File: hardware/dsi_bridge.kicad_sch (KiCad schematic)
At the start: 2 parts, among them J11 Conn_01x20_MountingPin, J12 Conn_01x20_MountingPin

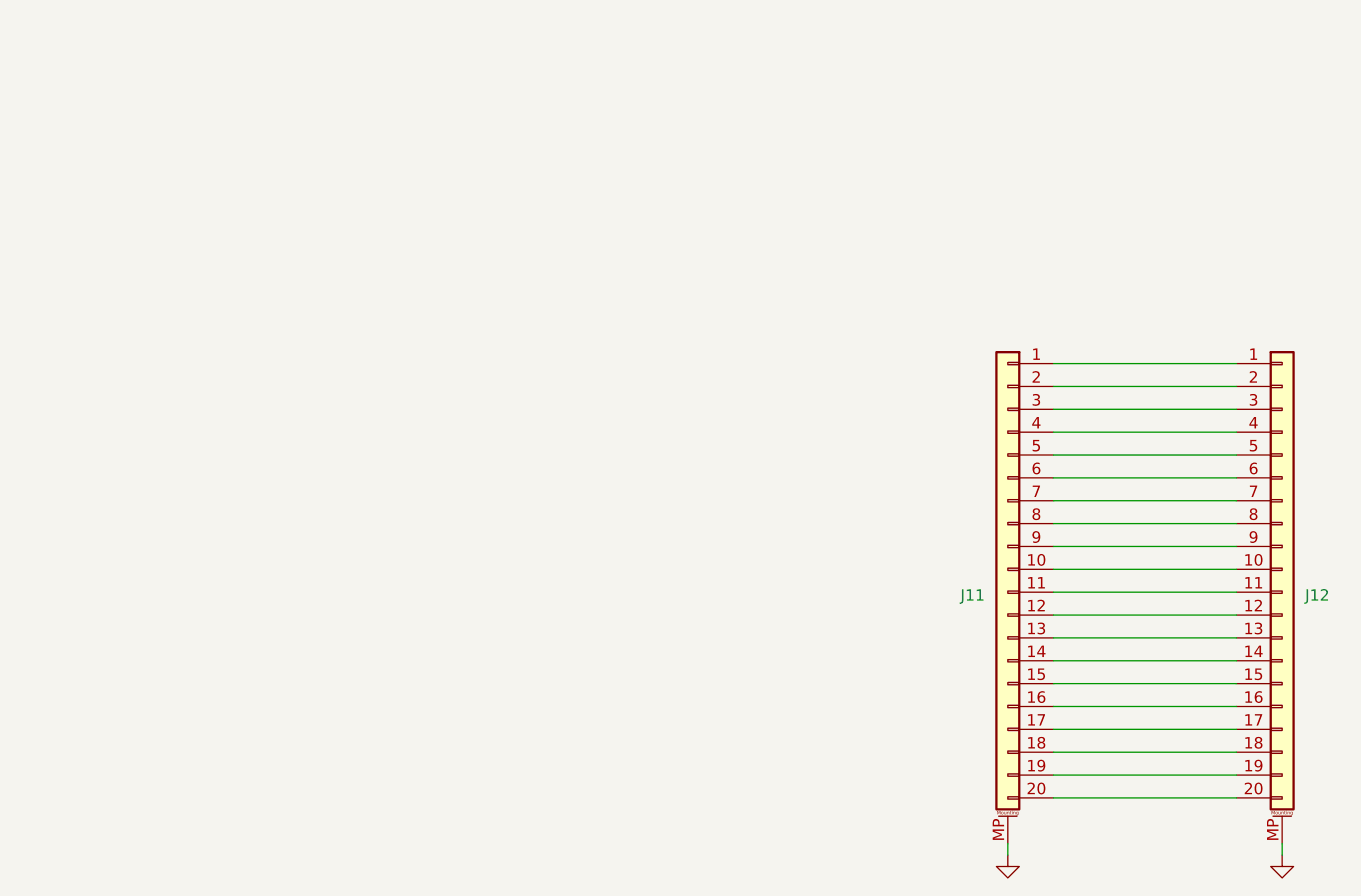
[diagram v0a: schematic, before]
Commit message: Passing DRC
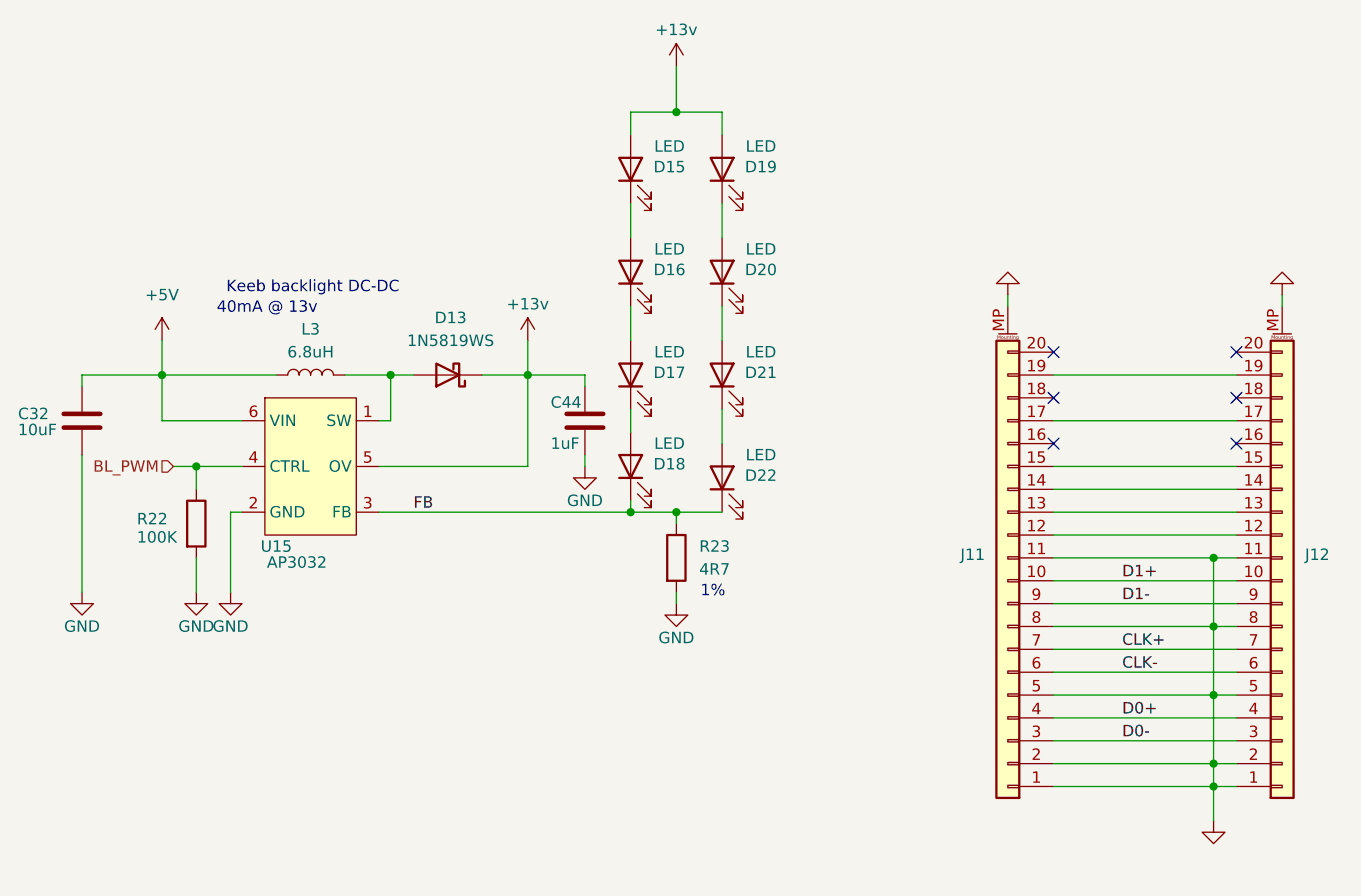
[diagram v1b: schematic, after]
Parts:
- added C32: 10uF, Capacitor_SMD:C_0603_1608Metric, symbol Device:C
- added C44: 1uF, Capacitor_SMD:C_0402_1005Metric, symbol Device:C
- added D13: 1N5819WS, Diode_SMD:D_SOD-323, symbol Device:D_Schottky
- added D15, D16, D17, D18, D19, D20, D21, D22: LED, keyboard_leds:LTW-010DCG, symbol Device:LED
- added L3: 6.8uH, Inductor_SMD:L_Vishay_IFSC-1515AH_4x4x1.8mm, symbol Device:L
- added R22: 100K, Resistor_SMD:R_0402_1005Metric, symbol Device:R
- added R23: 4R7, Resistor_SMD:R_0402_1005Metric, symbol Device:R
- added U15: AP3032, Package_TO_SOT_SMD:SOT-23-6_Handsoldering, symbol AP3032:AP3032
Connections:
- net GND: now also J11.1 (Pin_1), J11.11 (Pin_11), J11.2 (Pin_2), J11.5 (Pin_5), J11.8 (Pin_8), J12.1 (Pin_1), J12.11 (Pin_11), J12.2 (Pin_2), J12.5 (Pin_5), J12.8 (Pin_8), C32.2, C44.2, R22.2, R23.2, U15.2 (GND)
- net D1+: now reaches J11.10 (Pin_10), J12.10 (Pin_10)
- net at J11.16 (Pin_16): no longer J12.16 (Pin_16)
- net at J11.18 (Pin_18): no longer J12.18 (Pin_18)
- net at J11.20 (Pin_20): no longer J12.20 (Pin_20)
- net D0-: now reaches J11.3 (Pin_3), J12.3 (Pin_3)
- net D0+: now reaches J11.4 (Pin_4), J12.4 (Pin_4)
- net CLK-: now reaches J11.6 (Pin_6), J12.6 (Pin_6)
- net CLK+: now reaches J11.7 (Pin_7), J12.7 (Pin_7)
- net D1-: now reaches J11.9 (Pin_9), J12.9 (Pin_9)
- new net: D21.1 (K), D22.2 (A)
- new net: D20.1 (K), D21.2 (A)
- new net: D13.2 (A), L3.2, U15.1 (SW)
- new net: D17.1 (K), D18.2 (A)
- new net: D16.1 (K), D17.2 (A)
- new net: D15.1 (K), D16.2 (A)
- new net: D19.1 (K), D20.2 (A)
- new net +13v: C44.1, D13.1 (K), D15.2 (A), D19.2 (A), U15.5 (OV)
- new net +5V: C32.1, L3.1, U15.6 (VIN)
- new net BL_PWM: R22.1, U15.4 (CTRL)
- new net FB: D18.1 (K), D22.1 (K), R23.1, U15.3 (FB)
- no-connect marks 0 -> 6
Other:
- note added: "1%"
- note added: "40mA @ 13v"
- note added: "Keeb backlight DC-DC"
- moved on the sheet: J11, J12
